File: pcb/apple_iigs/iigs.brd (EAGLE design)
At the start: 81 x 45 mm, 16 parts, among them J1 ATX24RH

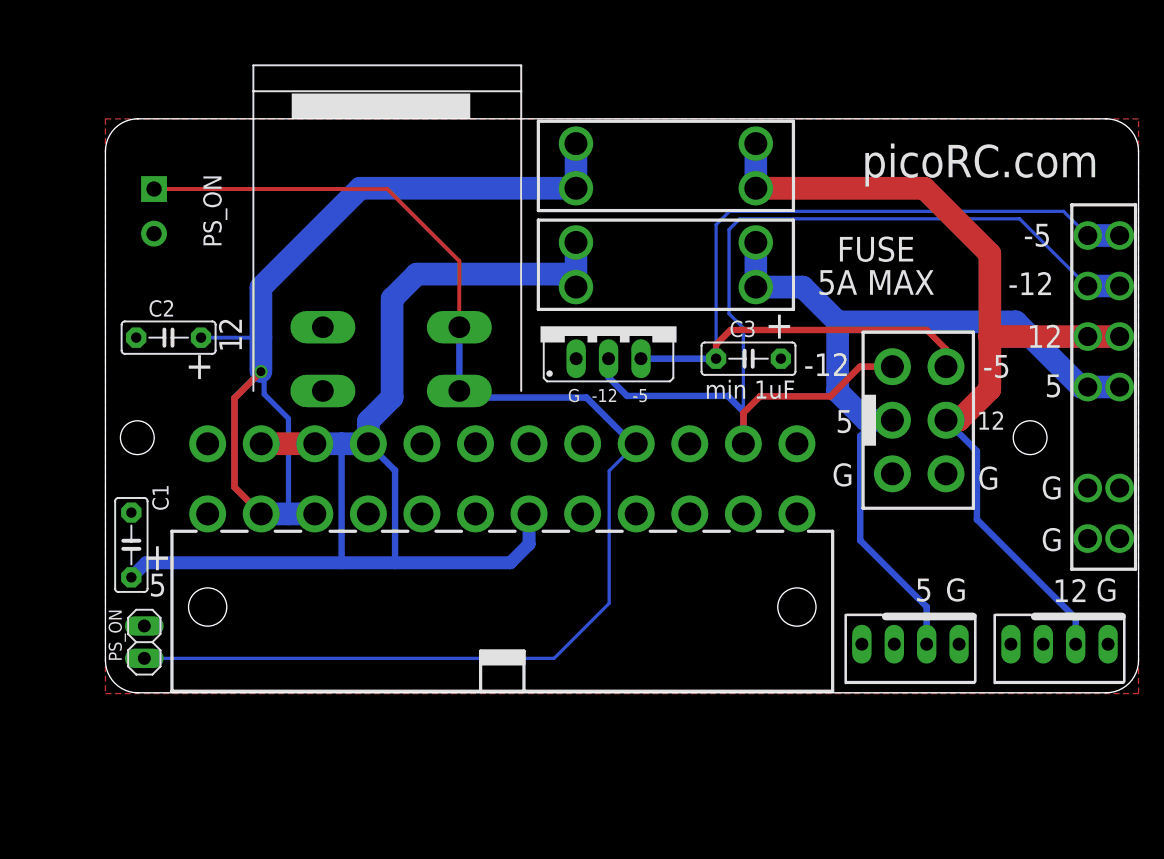
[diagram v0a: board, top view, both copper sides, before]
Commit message: added iigs
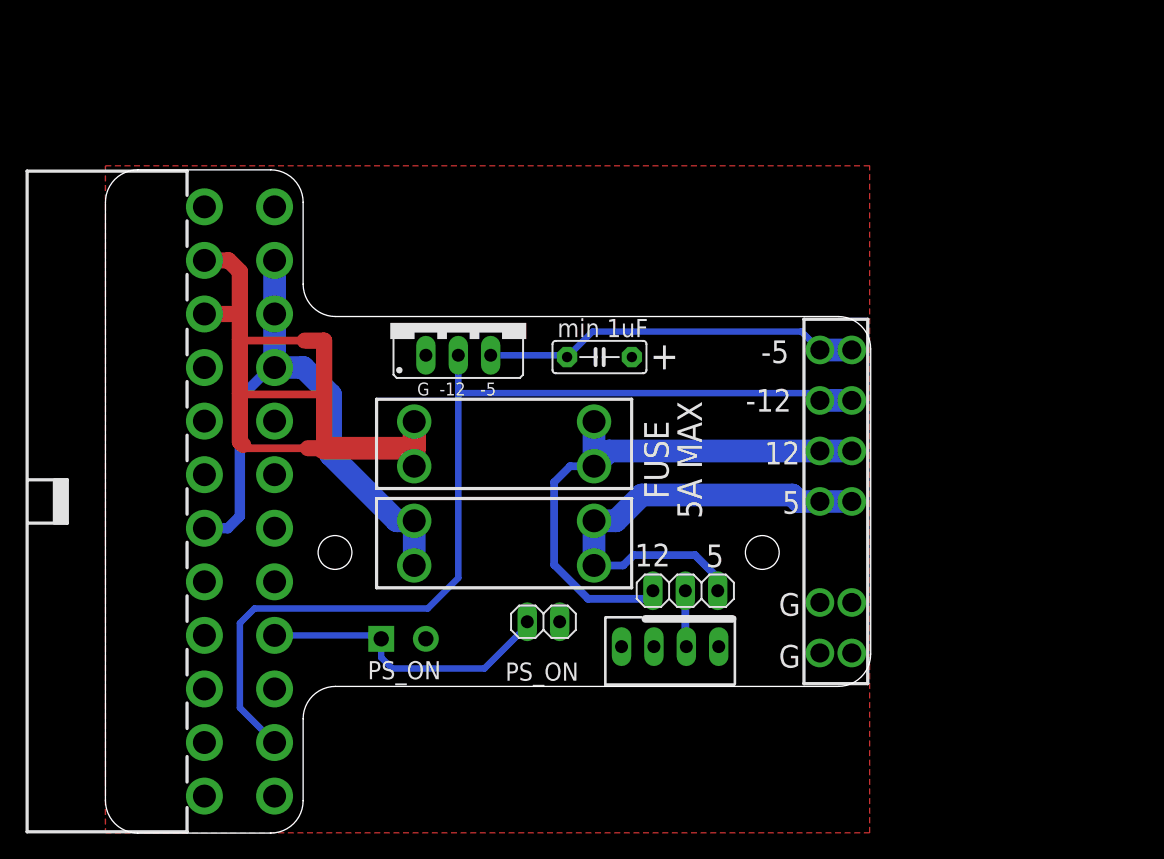
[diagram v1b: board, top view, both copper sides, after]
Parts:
- removed C1, C2: (no value), capacitor-wima:C5B2.5
- removed JP3: (no value), appleii:1X04
- removed U$3: ROCK_SW, atx4vc:ROCK_SWITCH
- removed U$6: APPLEII, atx4vc:APPLEII
- added JP2: (no value), pinhead:1X03
- J1: device macse:ATX24_RIGHT_ANGLE -> appleii:ATX24_RIGHT_ANGLE
- moved J7 39.5 mm to (21.6, 4.23), turned to 0 degrees
- moved JP1 31.3 mm to (34.3, 5.57), turned to 0 degrees
- moved J1 28.7 mm to (3.00, 15.0), turned to 270 degrees
- moved U$1 25.2 mm to (31.3, 11.7)
- moved U$2 25.2 mm to (31.3, 19.5)
- moved U$4 22.8 mm to (51.5, 11.0)
- moved U$7 22.8 mm to (57.3, 15.0)
- moved JP4 18.8 mm to (44.3, 3.62)
- moved U$5 17.9 mm to (18.0, 11.0)
- moved IC1 11.8 mm to (27.7, 29.0)
- moved C3 11.7 mm to (38.7, 26.3)
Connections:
- new net N$1: JP2.2, JP4.2
- net +12V: now also JP2.3; no longer JP3.2, U$6.4
- net +5V: now also JP2.1; no longer JP4.2, U$6.3
- net -12V: no longer U$6.5
- net -5V: no longer U$6.6
- net GND: no longer C1.2, C2.2, JP3.1, U$3.P$1, U$3.P$3, U$6.1, U$6.2
- net N$5: no longer U$3.P$2, U$3.P$4
- net N$6: no longer C1.1
- net N$8: no longer C2.1
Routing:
- net N$5: track 103.7 -> 23.4 mm
- net N$6: track 93.8 -> 46.7 mm
- net -5V: track 70.9 -> 29.8 mm
- net +5V: track 67.5 -> 36.5 mm
- net +12V: track 71.0 -> 43.4 mm
- net N$8: track 84.8 -> 60.1 mm, vias 1 -> 0
- net N$1: track 0.00 -> 4.41 mm
- net -12V: track 81.7 -> 77.6 mm
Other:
- board size 81 x 45 mm -> 60 x 52 mm
- board text added: "Apple IIgs PicoPSU Adaptor"
- board text removed: "Apple II / II Plus / IIe / IIgs PicoPSU Adaptor"
- board text removed: "picoRC.com"

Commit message: updated IIGS design
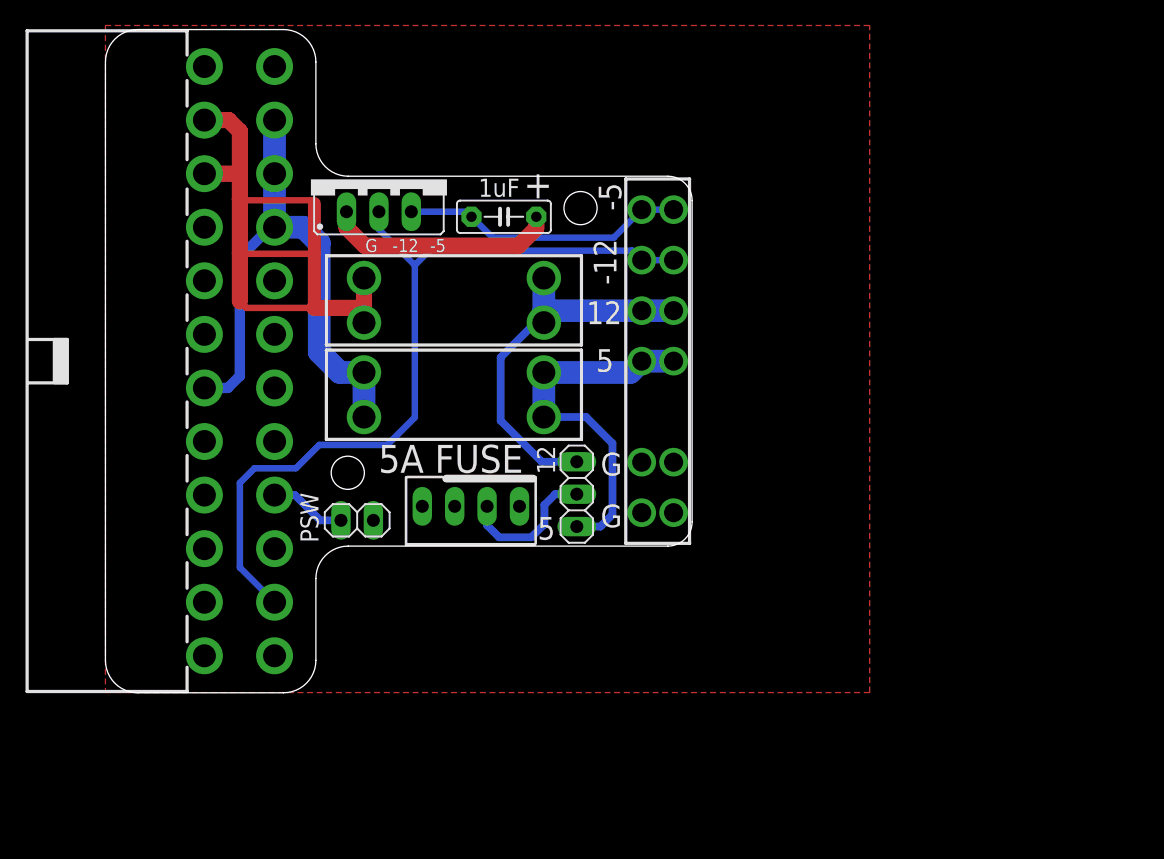
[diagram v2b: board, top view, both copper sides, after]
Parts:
- removed J7: (no value), atx_power_control:SCREWTERMINAL-3.5MM-2-NS
- removed U$4, U$5: M2.5_MOUNTING_HOLE, appleii:M3_MOUNTING_HOLE_PACK
- moved JP4 19.1 mm to (28.7, 14.6)
- moved U$7 17.8 mm to (43.3, 26.0)
- moved JP1 16.6 mm to (19.7, 13.5)
- moved C3 13.3 mm to (31.2, 37.3)
- moved IC1 12.9 mm to (21.4, 40.3)
- moved U$1 12.3 mm to (27.3, 23.4)
- moved U$2 11.9 mm to (27.3, 30.8)
- moved JP2 11.4 mm to (37.0, 15.6), turned to 90 degrees
- moved J1 11.0 mm to (3.00, 26.0)
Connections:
- net GND: no longer J7.2
- net N$5: no longer J7.1
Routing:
- net GND: track 0.00 -> 18.2 mm
- net N$5: track 23.4 -> 6.03 mm
- net -12V: track 77.6 -> 64.7 mm
- net +12V: track 43.4 -> 31.4 mm
- net +5V: track 36.5 -> 29.0 mm
- net -5V: track 29.8 -> 22.3 mm
- net N$8: track 60.1 -> 52.7 mm
- net N$1: track 4.41 -> 11.2 mm
- net N$6: track 46.7 -> 44.8 mm
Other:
- board size 60 x 52 mm -> 46 x 52 mm
- board text added: "1uF"
- board text added: "5A FUSE"
- board text added: "Apple IIGS PicoPSU Adaptor"
- board text added: "PD1 dekuNukem APR2023"
- board text added: "PSW"
- board text removed: "Apple IIgs PicoPSU Adaptor"
- board text removed: "FUSE 5A MAX"
- board text removed: "PS_ON"
- board text removed: "PT1 dekuNukem DEC 2022"
- board text removed: "min 1uF"
